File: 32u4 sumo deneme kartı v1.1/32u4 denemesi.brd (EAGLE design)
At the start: 100 x 100 mm, 136 parts, among them IC1 IC_555-SOIC8, IC2 LM2577S, IC3 LMV358MX, J1 AVR_SPI_PRG_6NS, Q2 SI3456BDVSOT-5-6, U1 TB6612FNG

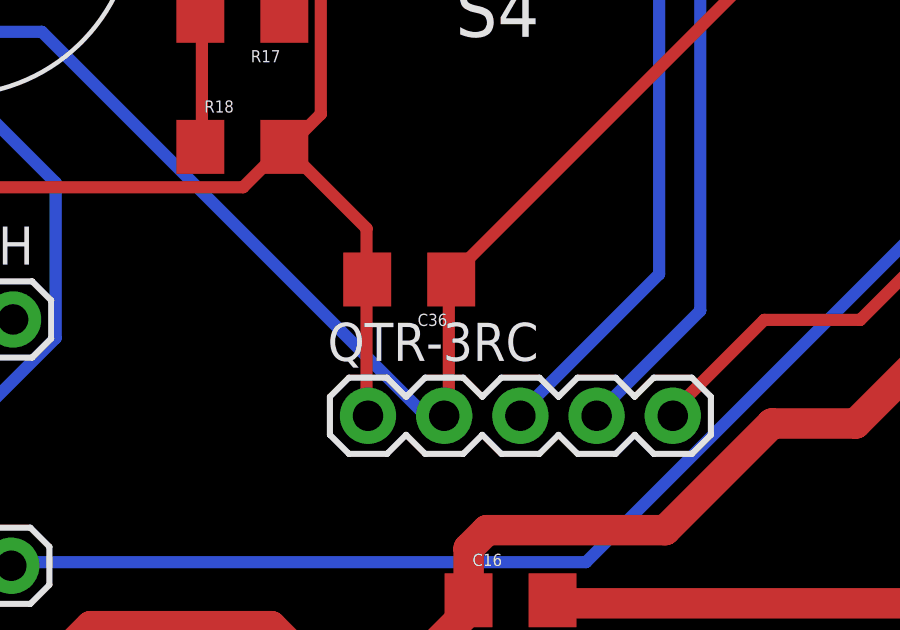
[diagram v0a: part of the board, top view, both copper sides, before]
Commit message: sws
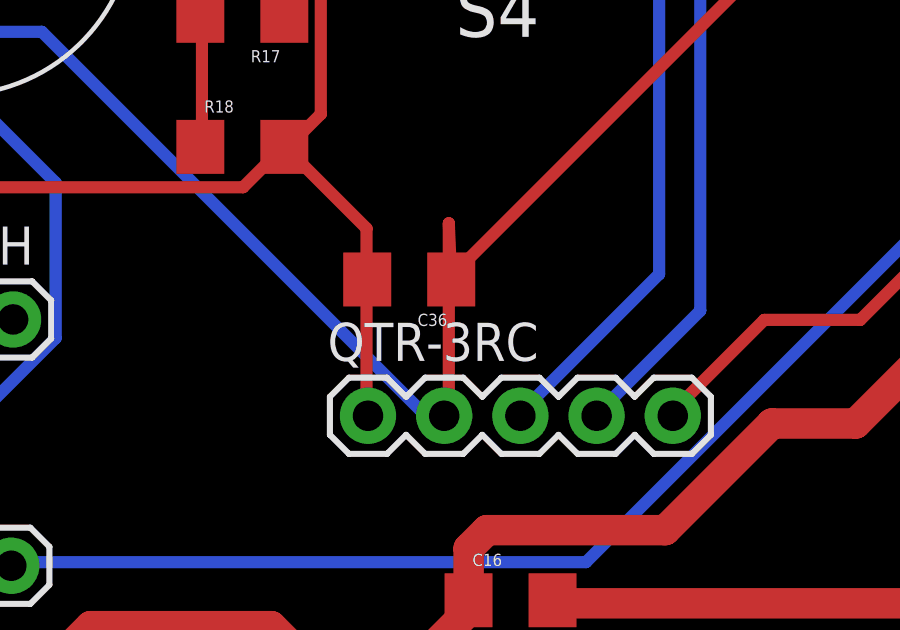
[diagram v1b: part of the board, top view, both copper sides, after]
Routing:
- net +5V: track 618.1 -> 621.9 mm
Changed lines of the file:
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@@
 <contactref element="C35" pad="1"/>
 <contactref element="C36" pad="1"/>
-<wire x1="24.384" y1="43.2816" x2="24.384" y2="47.3964" width="0.4064" layer="1"/>
+<wire x1="24.384" y1="43.2816" x2="24.384" y2="49.3964" width="0.4064" layer="1"/>
 <wire x1="24.2316" y1="43.1292" x2="24.384" y2="43.2816" width="0.4064" layer="1"/>
-<wire x1="24.384" y1="47.3964" x2="24.4632" y2="47.5234" width="0.4064" layer="1"/>
+<wire x1="24.384" y1="49.3964" x2="24.4632" y2="47.5234" width="0.4064" layer="1"/>
 <wire x1="24.2316" y1="43.1292" x2="24.23" y2="42.98" width="0.4064" layer="1"/>
 <wire x1="34.29" y1="57.4548" x2="34.29" y2="57.912" width="0.4064" layer="1"/>
